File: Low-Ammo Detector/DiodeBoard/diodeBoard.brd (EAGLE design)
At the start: 8 x 9 mm, 2 parts

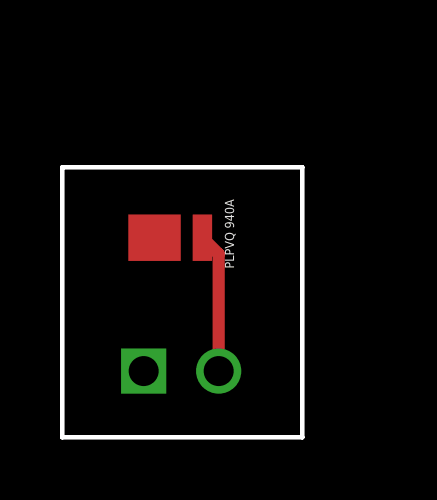
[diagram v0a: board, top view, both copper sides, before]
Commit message: added changes since repo changes
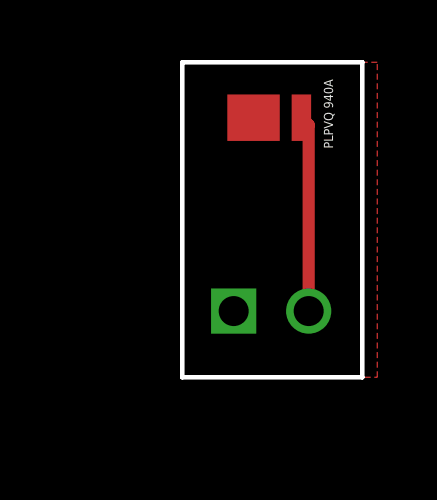
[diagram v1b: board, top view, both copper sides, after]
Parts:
- moved U$2 5.19 mm to (4.30, 7.87)
- moved U$1 3.61 mm to (1.71, 2.21)
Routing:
- net 1.5V: track 4.67 -> 6.55 mm
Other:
- board size 8 x 9 mm -> 6 x 10.5 mm
- board text added: "Purdue Robomaster Diode Board By Henry Silva"
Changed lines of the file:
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@@
 <setting verticaltext="up"/>
 </settings>
-<grid distance="39.3700787" unitdist="mil" unit="mil" style="lines" multiple="1" display="yes" altdistance="5" altunitdist="mil" altunit="mil"/>
+<grid distance="0.1" unitdist="mm" unit="mm" style="lines" multiple="1" display="yes" altdistance="5" altunitdist="mil" altunit="mil"/>
 <layers>
 <layer number="1" name="Top" color="4" fill="1" visible="yes" active="yes"/>
@@
 <layer number="21" name="tPlace" color="7" fill="1" visible="yes" active="yes"/>
 <layer number="22" name="bPlace" color="7" fill="1" visible="yes" active="yes"/>
-<layer number="23" name="tOrigins" color="15" fill="1" visible="yes" active="yes"/>
-<layer number="24" name="bOrigins" color="15" fill="1" visible="yes" active="yes"/>
-<layer number="25" name="tNames" color="7" fill="1" visible="yes" active="yes"/>
-<layer number="26" name="bNames" color="7" fill="1" visible="yes" active="yes"/>
-<layer number="27" name="tValues" color="7" fill="1" visible="yes" active="yes"/>
-<layer number="28" name="bValues" color="7" fill="1" visible="yes" active="yes"/>
+<layer number="23" name="tOrigins" color="15" fill="1" visible="no" active="yes"/>
+<layer number="24" name="bOrigins" color="15" fill="1" visible="no" active="yes"/>
+<layer number="25" name="tNames" color="7" fill="1" visible="no" active="yes"/>
+<layer number="26" name="bNames" color="7" fill="1" visible="no" active="yes"/>
+<layer number="27" name="tValues" color="7" fill="1" visible="no" active="yes"/>
+<layer number="28" name="bValues" color="7" fill="1" visible="no" active="yes"/>
 <layer number="29" name="tStop" color="7" fill="3" visible="no" active="yes"/>
 <layer number="30" name="bStop" color="7" fill="6" visible="no" active="yes"/>
@@
 <layer number="37" name="tTest" color="7" fill="1" visible="no" active="yes"/>
 <layer number="38" name="bTest" color="7" fill="1" visible="no" active="yes"/>
-<layer number="39" name="tKeepout" color="4" fill="11" visible="yes" active="yes"/>
-<layer number="40" name="bKeepout" color="1" fill="11" visible="yes" active="yes"/>
-<layer number="41" name="tRestrict" color="4" fill="10" visible="yes" active="yes"/>
-<layer number="42" name="bRestrict" color="1" fill="10" visible="yes" active="yes"/>
-<layer number="43" name="vRestrict" color="2" fill="10" visible="yes" active="yes"/>
+<layer number="39" name="tKeepout" color="4" fill="11" visible="no" active="yes"/>
+<layer number="40" name="bKeepout" color="1" fill="11" visible="no" active="yes"/>
+<layer number="41" name="tRestrict" color="4" fill="10" visible="no" active="yes"/>
+<layer number="42" name="bRestrict" color="1" fill="10" visible="no" active="yes"/>
+<layer number="43" name="vRestrict" color="2" fill="10" visible="no" active="yes"/>
 <layer number="44" name="Drills" color="7" fill="1" visible="no" active="yes"/>
 <layer number="45" name="Holes" color="7" fill="1" visible="no" active="yes"/>
 <layer number="46" name="Milling" color="3" fill="1" visible="no" active="yes"/>
 <layer number="47" name="Measures" color="7" fill="1" visible="no" active="yes"/>
-<layer number="48" name="Document" color="7" fill="1" visible="yes" active="yes"/>
-<layer number="49" name="Reference" color="7" fill="1" visible="yes" active="yes"/>
+<layer number="48" name="Document" color="7" fill="1" visible="no" active="yes"/>
+<layer number="49" name="Reference" color="7" fill="1" visible="no" active="yes"/>
 <layer number="50" name="dxf" color="7" fill="1" visible="no" active="no"/>
-<layer number="51" name="tDocu" color="7" fill="1" visible="yes" active="yes"/>
-<layer number="52" name="bDocu" color="7" fill="1" visible="yes" active="yes"/>
+<layer number="51" name="tDocu" color="7" fill="1" visible="no" active="yes"/>
+<layer number="52" name="bDocu" color="7" fill="1" visible="no" active="yes"/>
 <layer number="53" name="tGND_GNDA" color="7" fill="9" visible="no" active="no"/>
 <layer number="54" name="bGND_GNDA" color="1" fill="9" visible="no" active="no"/>
@@
 <layer number="112" name="tSilk" color="7" fill="1" visible="no" active="yes"/>
 <layer number="113" name="ReferenceLS" color="7" fill="1" visible="no" active="no"/>
-<layer number="114" name="Badge_Outline" color="7" fill="1" visible="yes" active="yes"/>
-<layer number="115" name="ReferenceISLANDS" color="7" fill="1" visible="yes" active="yes"/>
+<layer number="114" name="Badge_Outline" color="7" fill="1" visible="no" active="yes"/>
+<layer number="115" name="ReferenceISLANDS" color="7" fill="1" visible="no" active="yes"/>
 <layer number="116" name="Patch_BOT" color="9" fill="4" visible="no" active="yes"/>
 <layer number="118" name="Rect_Pads" color="7" fill="1" visible="no" active="no"/>
@@
 <layer number="127" name="_tValues" color="7" fill="1" visible="no" active="yes"/>
 <layer number="128" name="_bValues" color="7" fill="1" visible="no" active="yes"/>
-<layer number="129" name="Mask" color="7" fill="1" visible="yes" active="yes"/>
+<layer number="129" name="Mask" color="7" fill="1" visible="no" active="yes"/>
 <layer number="131" name="tAdjust" color="7" fill="1" visible="no" active="yes"/>
 <layer number="132" name="bAdjust" color="7" fill="1" visible="no" active="yes"/>
@@
 <layer number="223" name="223bmp" color="24" fill="1" visible="no" active="no"/>
 <layer number="224" name="224bmp" color="25" fill="1" visible="no" active="no"/>
-<layer number="225" name="225bmp" color="7" fill="1" visible="yes" active="yes"/>
-<layer number="226" name="226bmp" color="7" fill="1" visible="yes" active="yes"/>
-<layer number="227" name="227bmp" color="7" fill="1" visible="yes" active="yes"/>
-<layer number="228" name="228bmp" color="7" fill="1" visible="yes" active="yes"/>
-<layer number="229" name="229bmp" color="7" fill="1" visible="yes" active="yes"/>
-<layer number="230" name="230bmp" color="7" fill="1" visible="yes" active="yes"/>
+<layer number="225" name="225bmp" color="7" fill="1" visible="no" active="yes"/>
+<layer number="226" name="226bmp" color="7" fill="1" visible="no" active="yes"/>
+<layer number="227" name="227bmp" color="7" fill="1" visible="no" active="yes"/>
+<layer number="228" name="228bmp" color="7" fill="1" visible="no" active="yes"/>
+<layer number="229" name="229bmp" color="7" fill="1" visible="no" active="yes"/>
+<layer number="230" name="230bmp" color="7" fill="1" visible="no" active="yes"/>
 <layer number="231" name="Eagle3D_PG1" color="7" fill="1" visible="no" active="no"/>
 <layer number="232" name="Eagle3D_PG2" color="7" fill="1" visible="no" active="no"/>
@@
 <layer number="251" name="SMDround" color="7" fill="1" visible="no" active="no"/>
 <layer number="254" name="cooling" color="7" fill="1" visible="no" active="yes"/>
-<layer number="255" name="routoute" color="7" fill="1" visible="yes" active="yes"/>
+<layer number="255" name="routoute" color="7" fill="1" visible="no" active="yes"/>
 </layers>
 <board>
 <plain>
-<wire x1="-4" y1="-2" x2="4" y2="-2" width="0.1524" layer="20"/>
-<wire x1="4" y1="-2" x2="4" y2="7" width="0.1524" layer="20"/>
-<wire x1="4" y1="7" x2="-4" y2="7" width="0.1524" layer="20"/>
-<wire x1="-4" y1="7" x2="-4" y2="-2" width="0.1524" layer="20"/>
+<wire x1="0" y1="0" x2="6" y2="0" width="0.1524" layer="20"/>
+<wire x1="6" y1="0" x2="6" y2="10.5" width="0.1524" layer="20"/>
+<wire x1="6" y1="10.5" x2="0" y2="10.5" width="0.1524" layer="20"/>
+<wire x1="0" y1="10.5" x2="0" y2="0" width="0.1524" layer="20"/>
+<text x="5.5" y="4.6" size="0.4064" layer="22" font="vector" rot="MR0">Purdue Robomaster
+Diode Board
+By Henry Silva</text>
 </plain>
 <attributes>
@@
 </autorouter>
 <elements>
-<element name="U$1" library="_HenrySilva" package="2PIN" value="2PIN" x="-1.287" y="0.207" smashed="yes"/>
-<element name="U$2" library="_HenrySilva" package="PLPVQ940A" value="PLPVQ940A" x="1" y="3.873" smashed="yes" rot="R90"/>
+<element name="U$1" library="_HenrySilva" package="2PIN" value="2PIN" x="1.713" y="2.207" smashed="yes"/>
+<element name="U$2" library="_HenrySilva" package="PLPVQ940A" value="PLPVQ940A" x="4.3" y="7.873" smashed="yes" rot="R90"/>
 </elements>
 <signals>
@@
 <contactref element="U$1" pad="P$2"/>
 <contactref element="U$2" pad="P$1"/>
-<wire x1="1.213" y1="0.207" x2="1.213" y2="4.11" width="0.4064" layer="1"/>
-<wire x1="1.213" y1="4.11" x2="0.67" y2="4.653" width="0.4064" layer="1"/>
+<wire x1="4.213" y1="2.207" x2="4.213" y2="8.41" width="0.4064" layer="1"/>
+<wire x1="4.213" y1="8.41" x2="3.97" y2="8.653" width="0.4064" layer="1"/>
 </signal>
 <signal name="GND">
@@
 <contactref element="U$2" pad="P$2"/>
 <polygon width="0.4064" layer="1">
-<vertex x="-4" y="7"/>
-<vertex x="-4" y="-2"/>
-<vertex x="4" y="-2"/>
-<vertex x="4" y="7"/>
+<vertex x="0" y="10.5"/>
+<vertex x="0" y="0"/>
+<vertex x="6.5" y="0"/>
+<vertex x="6.5" y="10.5"/>
 </polygon>
 </signal>
@@
 <mfgpreviewcolor name="substratecolor" color="0xFF786E46"/>
 </mfgpreviewcolors>
+<errors>
+</errors>
 </board>
 </drawing>
+<compatibility>
+<note version="6.3" minversion="6.2.2" severity="warning">
+Since Version 6.2.2 text objects can contain more than one line,
+which will not be processed correctly with this version.
+</note>
+</compatibility>
 </eagle>
